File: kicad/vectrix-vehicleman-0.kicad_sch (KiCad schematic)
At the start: 39 parts, among them J4 Molex_104031-0811, Q1 BSS138, Q2 BSS138, Q4 Q_PMOS_30V_5.5A_SOT23, U1 ESP32-WROVER-IE-N16R8, U10 CH340C, U16 TPS3808DBV, Y1 32.768kHz 12.5pF

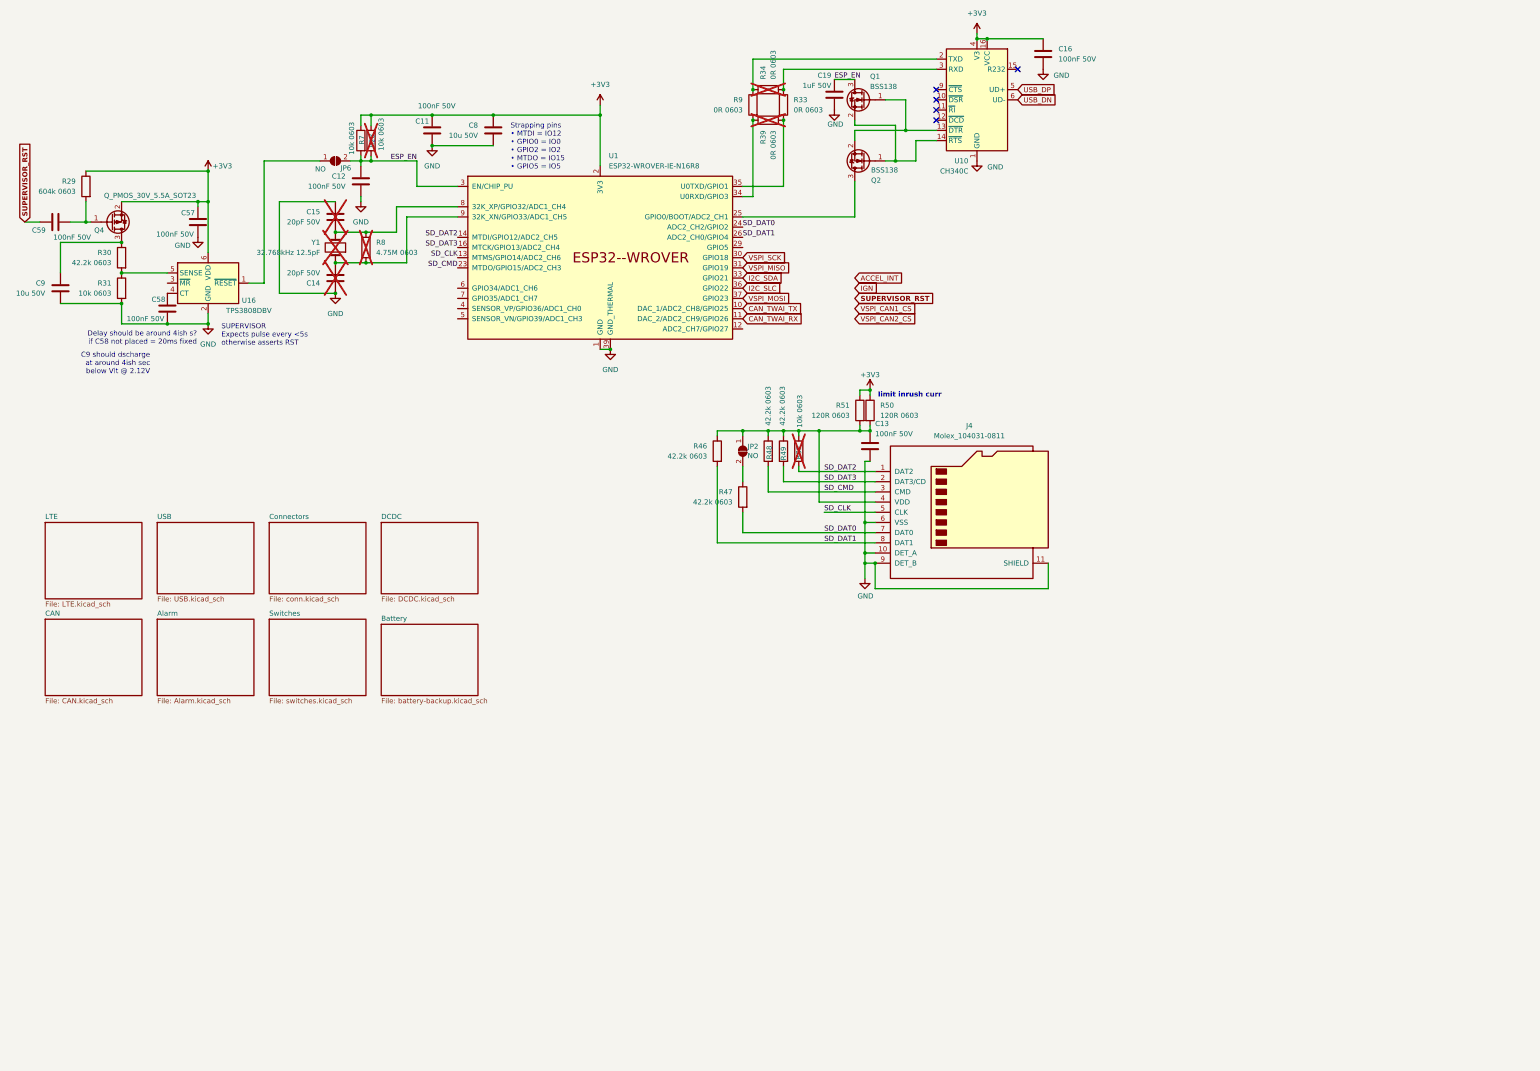
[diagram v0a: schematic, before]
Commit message: sch done-ish
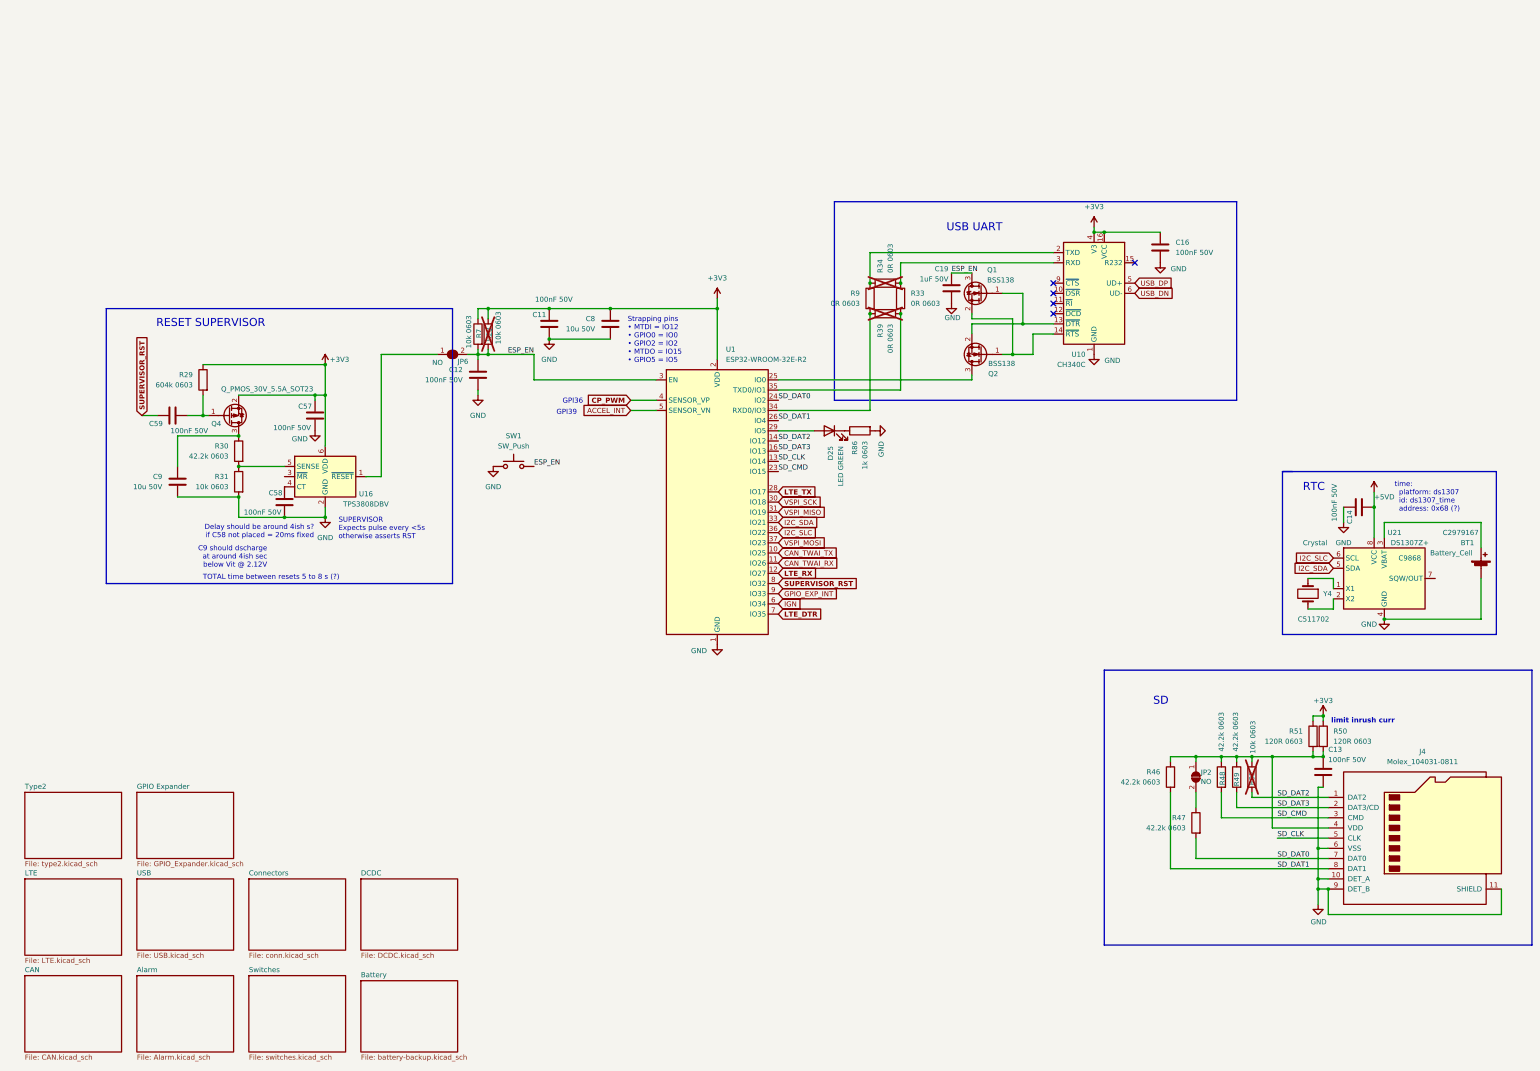
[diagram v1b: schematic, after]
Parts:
- removed C15: 20pF 50V, Capacitor_SMD:C_0603_1608Metric, symbol Device:C
- removed R8: 4.75M 0603, Resistor_SMD:R_0603_1608Metric, symbol Device:R
- removed U1: ESP32-WROVER-IE-N16R8, PCM_Espressif:ESP32-WROVER-E, symbol PCM_Espressif:ESP32-WROVER-E
- removed Y1: 32.768kHz 12.5pF, Crystal:Crystal_SMD_HC49-SD, symbol Device:Crystal
- added BT1: Battery_Cell, Battery:BatteryHolder_MYOUNG_BS-07-A1BJ001_CR2032, symbol Device:Battery_Cell
- added D25: LED GREEN, LED_SMD:LED_0805_2012Metric, symbol Device:LED
- added R86: 1k 0603, Resistor_SMD:R_0603_1608Metric, symbol Device:R
- added SW1: SW_Push, Button_Switch_THT:SW_PUSH_6mm, symbol Switch:SW_Push
- added U1: ESP32-WROOM-32E-R2, RF_Module:ESP32-WROOM-32D, symbol RF_Module:ESP32-WROOM-32E-R2
- added U21: DS1307Z+, Package_SO:SOIC-8_3.9x4.9mm_P1.27mm, symbol Timer_RTC:DS1307Z+
- added Y4: Crystal, Crystal:Crystal_DS26_D2.0mm_L6.0mm_Horizontal, symbol Device:Crystal
- C14: value 20pF 50V -> 100nF 50V; LCSC C105621 -> C14663; now fitted
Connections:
- net +3V3: now also U1.2 (VDD)
- net ACCEL_INT: now also U1.5 (SENSOR_VN)
- net CAN_TWAI_RX: now also U1.11 (IO26)
- net CAN_TWAI_TX: now also U1.10 (IO25)
- net ESP_EN: now also SW1.2, U1.3 (EN)
- net GND: now also BT1.2 (-), R86.2, SW1.1, U1.1 (GND), U1.15 (GND), U1.38 (GND), U1.39 (GND), U21.4 (GND)
- net I2C_SDA: now also U1.33 (IO21), U21.5 (SDA)
- net I2C_SLC: now also U1.36 (IO22), U21.6 (SCL)
- net IGN: now also U1.6 (IO34)
- net SD_CLK: now also U1.13 (IO14)
- net SD_CMD: now also U1.23 (IO15)
- net SD_DAT0: now also U1.24 (IO2)
- net SD_DAT1: now also U1.26 (IO4)
- net SD_DAT2: now also U1.14 (IO12)
- net SD_DAT3: now also U1.16 (IO13)
- net SUPERVISOR_RST: now also U1.8 (IO32)
- net VSPI_MISO: now also U1.31 (IO19)
- net VSPI_MOSI: now also U1.37 (IO23)
- net VSPI_SCK: now also U1.30 (IO18)
- net at R39.1, R9.2: now also U1.34 (RXD0/IO3)
- net at R33.2, R39.2: now also U1.35 (TXD0/IO1)
- net at Q2.3 (D): now also U1.25 (IO0)
- net +5VD: now reaches C14.2
- net +5VD: now also U21.8 (VCC)
- new net: BT1.1 (+), U21.3 (VBAT)
- new net: D25.1 (K), R86.1
- new net: D25.2 (A), U1.29 (IO5)
- new net: U21.1 (X1), Y4.1
- new net: U21.2 (X2), Y4.2
- new net CP_PWM: U1.4 (SENSOR_VP)
- new net GPIO_EXP_INT: U1.9 (IO33)
- new net LTE_DTR: U1.7 (IO35)
- new net LTE_RX: U1.12 (IO27)
- new net LTE_TX: U1.28 (IO17)
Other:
- added sheet GPIO Expander (GPIO_Expander.kicad_sch)
- added sheet Type2 (type2.kicad_sch)
- note added: "GPI36"
- note added: "GPI39"
- note added: "RESET SUPERVISOR"
- note added: "RTC"
- note added: "SD"
- note added: "TOTAL time between resets 5 to 8 s (?)"
- note added: "USB UART"
- note added: "time: platform: ds1307 id: ds1307_time address: 0x68 (?)"
- company: (none) -> ©CC-BY-NC
- title: (none) -> VehicleMan
- moved on the sheet: C11, C12, C13, C16, C19, C57, C58, C59, C8, C9, J4, JP2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

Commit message: WIP
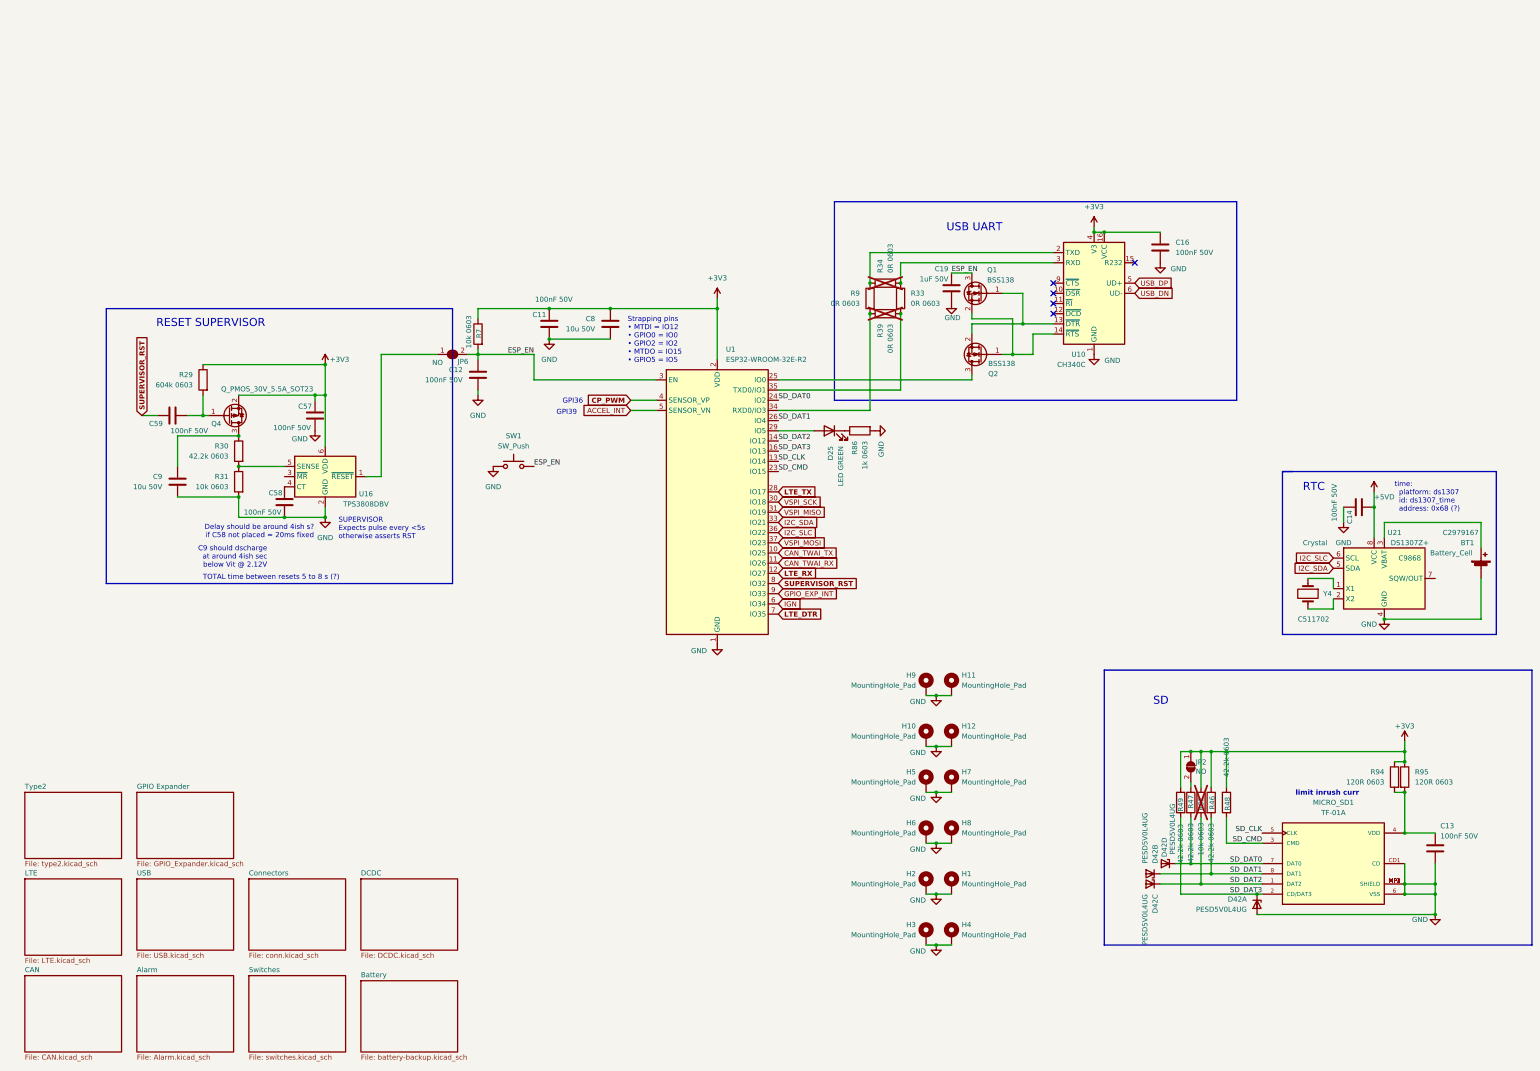
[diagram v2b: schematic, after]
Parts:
- removed J4: Molex_104031-0811, Connector_Card:microSD_HC_Molex_104031-0811, symbol Connector:Micro_SD_Card_Det_Hirose_DM3AT
- removed R28: 10k 0603, Resistor_SMD:R_0603_1608Metric, symbol Device:R
- removed R50, R51: 120R 0603, Resistor_SMD:R_0603_1608Metric, symbol Device:R
- added D42: PESD5V0L4UG, Package_TO_SOT_SMD:SOT-353_SC-70-5, symbol Power_Protection:PESD5V0L4UG
- added H1, H10, H11, H12, H2, H3, H4, H5, H6, H7, H8, H9: MountingHole_Pad, MountingHole:MountingHole_3.2mm_M3_DIN965_Pad_TopBottom, symbol Mechanical:MountingHole_Pad
- added MICRO_SD1: TF-01A, vehicle-manager:TF-01A, symbol vehicle-manager:TF-01A
- added R94, R95: 120R 0603, Resistor_SMD:R_0603_1608Metric, symbol Device:R
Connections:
- net +3V3: now also JP2.1 (A), R32.1, R46.1, R48.1, R49.1, R94.1, R95.1
- net GND: now also D42.2 (A), H1.1, H10.1, H11.1, H12.1, H2.1, H3.1, H4.1, H5.1, H6.1, H7.1, H8.1, H9.1, MICRO_SD1.6 (VSS), MICRO_SD1.CD1 (CD), MICRO_SD1.MP1 (SHIELD), MICRO_SD1.MP2 (SHIELD), MICRO_SD1.MP3 (SHIELD), MICRO_SD1.MP4 (SHIELD)
- net SD_CLK: now also MICRO_SD1.5 (CLK)
- net SD_CMD: now also MICRO_SD1.3 (CMD)
- net SD_DAT0: now also D42.5 (K4), MICRO_SD1.7 (DAT0)
- net SD_DAT1: now also D42.3 (K2), MICRO_SD1.8 (DAT1)
- net SD_DAT2: now also D42.4 (K3), MICRO_SD1.1 (DAT2)
- net SD_DAT3: now also D42.1 (K1), MICRO_SD1.2 (CD/DAT3)
- new net: C13.1, MICRO_SD1.4 (VDD), R94.2, R95.2
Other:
- moved on the sheet: C13, JP2, R32, R46, R47, R48, R49
